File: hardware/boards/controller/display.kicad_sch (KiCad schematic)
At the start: 13 parts, among them J3 01x06, J4 01x02, U4 ILI9341

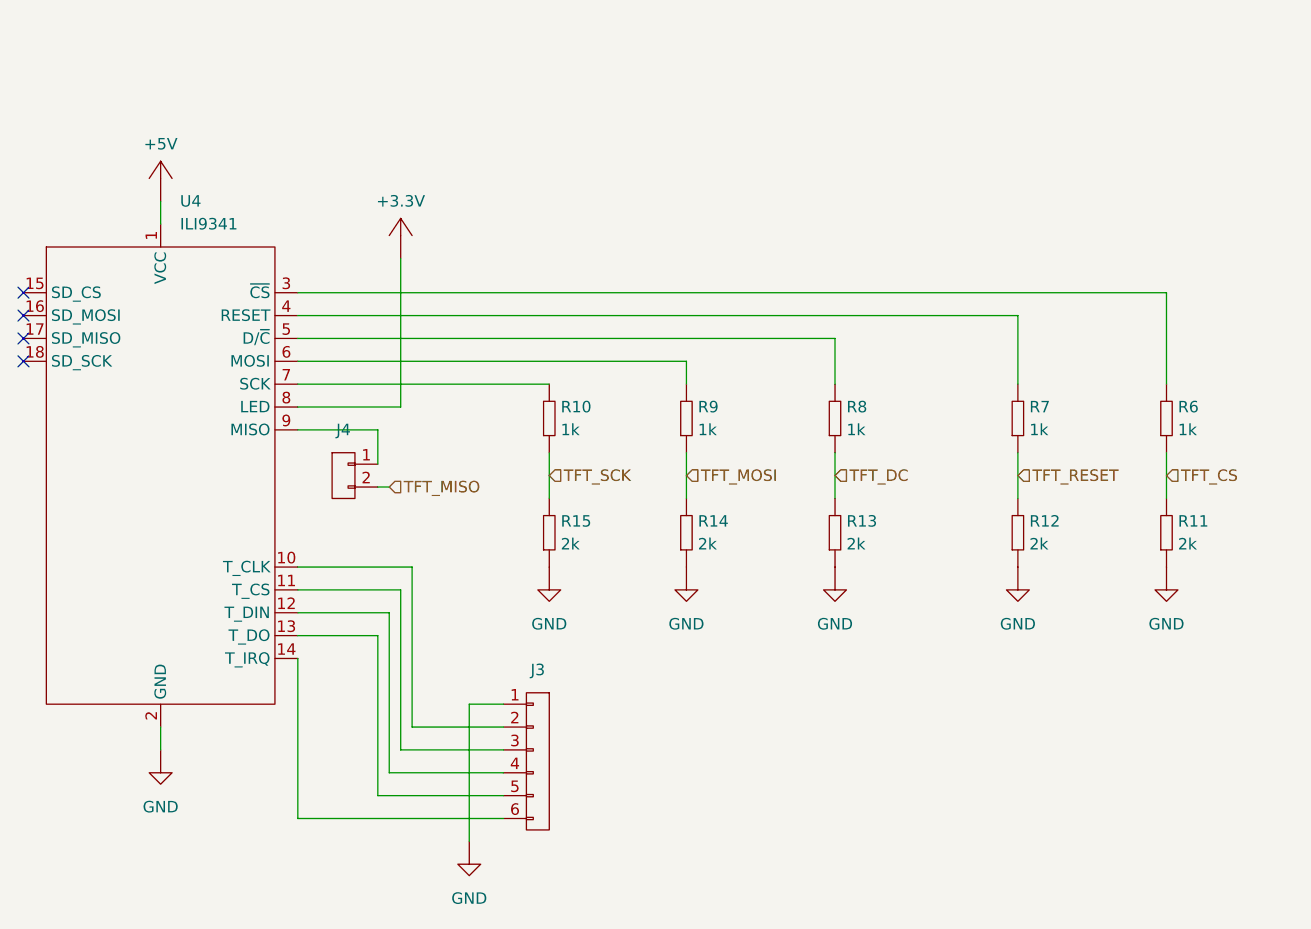
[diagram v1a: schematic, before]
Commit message: new version for pcb controller
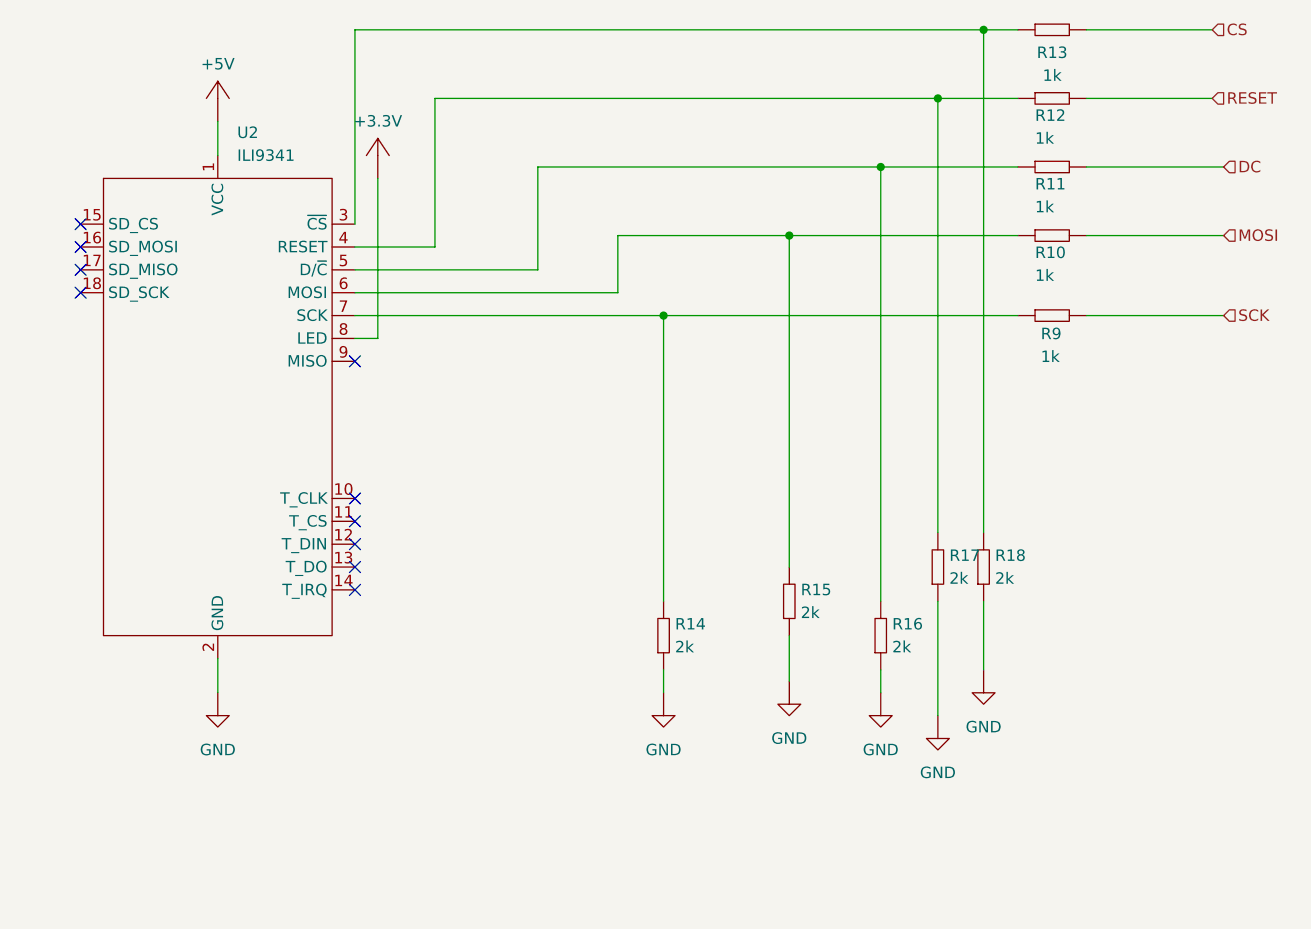
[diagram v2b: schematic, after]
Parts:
- removed J3: 01x06, connector:Pin_01x06, symbol connector:Pin_01x06
- removed J4: 01x02, connector:Pin_01x02, symbol connector:Pin_01x02
- U2: renamed from U4; Manufacturer (none) -> Adafruit
- renumbered R9 to R10, R8 to R11, R7 to R12, R6 to R13, R15 to R14, R14 to R15, R13 to R16, R12 to R17, R11 to R18, R10 to R9
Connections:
- net TFT_CS is gone; now on an unnamed net: R13.1, R18.2
- net TFT_DC is gone; now on an unnamed net: R11.1, R16.2
- net TFT_MOSI is gone; now on an unnamed net: R10.1, R15.2
- net TFT_RESET is gone; now on an unnamed net: R12.1, R17.2
- net TFT_SCK is gone; now on an unnamed net: R14.2, R9.1
- net at U2.7 (SCK): no longer R9.2
- net at U2.6 (MOSI): no longer R10.2
- net at U2.4 (RESET): no longer R12.2
- net at U2.5 (D/~{C}): no longer R11.2
- net at U2.3 (~{CS}): no longer R13.2
- new net CS: R13.2
- new net DC: R11.2
- new net MOSI: R10.2
- new net RESET: R12.2
- new net SCK: R9.2
- no-connect marks 4 -> 10
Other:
- moved on the sheet: R10, R11, R12, R13, R14, R15, R16, R17, R18, R9, U2
